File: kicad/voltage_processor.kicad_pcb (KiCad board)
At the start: 2 copper layers, 113 x 110 mm, 222 parts, among them IC1 DG212BDY, IC2 DG212BDY, IC3 DG212BDY, IC4 DG212BDY, J1 ATNVRT_IN_BOTTOM, J10 OUTPUT, J11 CROSSFADE_CV, J12 CROSSFADE_A, J13 CROSSFADE_B, J14 OUTPUT, J15 Conn_01x10_Male, J16 Conn_01x10_Male, J17 30310-6002HB, J2 ATNVRT_IN_BOTTOM, J3 Conn_01x16_Female, J4 Conn_01x10_Female, J5 Conn_01x16_Male, J6 Conn_01x10_Female, J7 CROSSFADE_CV, J8 CROSSFADE_A, J9 CROSSFADE_B, Q1 3906, Q2 3904, Q3 3906, Q4 3904, U1 OPA4134, U10 SSI2164, U11 OPA4134, U2 L78L05, U4 OPA4134, U5 OPA4134, U6 SSI2164, U8 OPA4134, U9 OPA4134

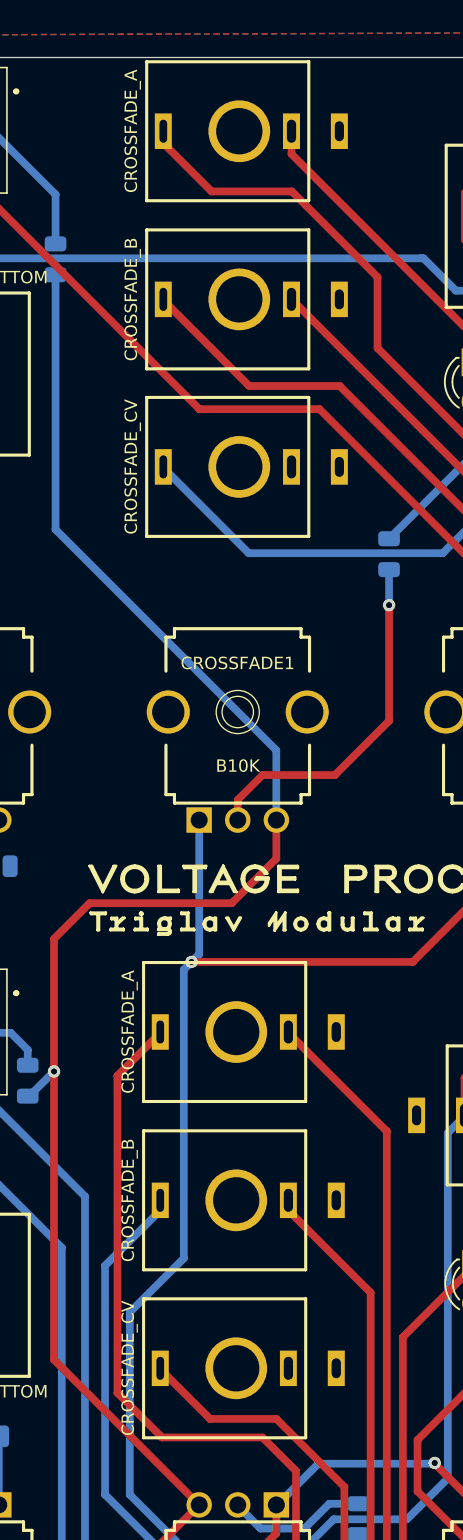
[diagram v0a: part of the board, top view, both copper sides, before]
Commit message: fixes
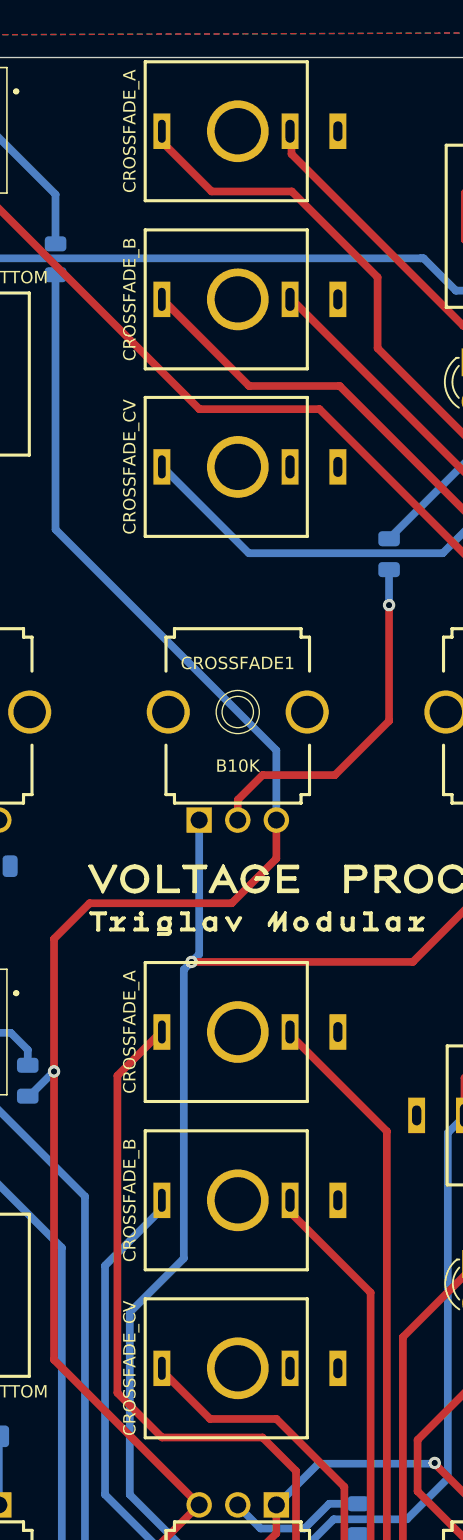
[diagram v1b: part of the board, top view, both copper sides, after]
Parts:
- moved J11 0.11 mm to (123.1, 128.3)
- moved J12 0.11 mm to (123.1, 106.5)
- moved J13 0.11 mm to (123.1, 117.4)
- moved J7 0.09 mm to (123.1, 69.9)
- moved J8 0.09 mm to (123.1, 48.2)
- moved J9 0.09 mm to (123.1, 59.1)
